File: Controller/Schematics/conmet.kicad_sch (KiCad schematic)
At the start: 14 parts, among them Q1 FQU20N06L, U1 RGBW_Led_Strip, U2 MP1584EN, U3 JS202011AQN, U4 VL53L1X

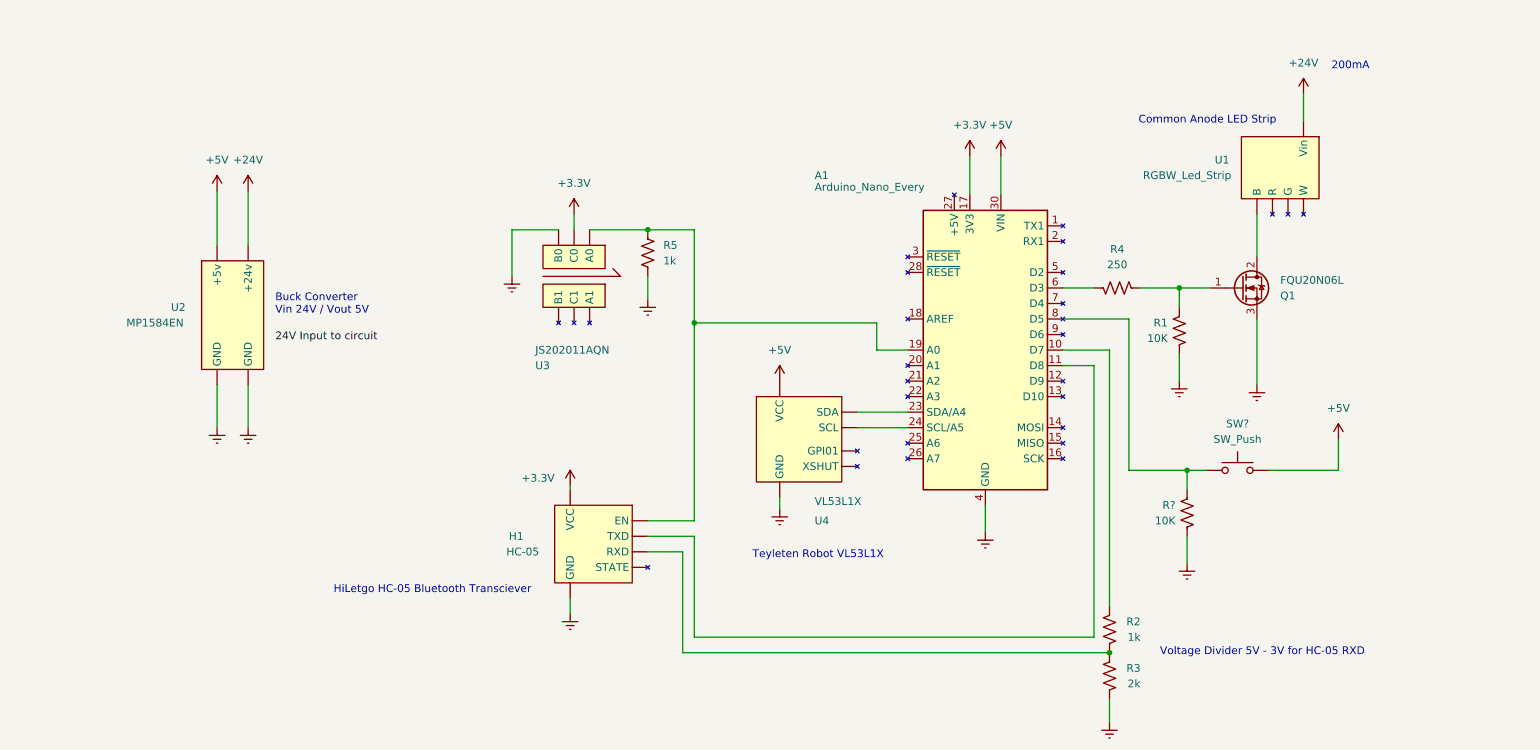
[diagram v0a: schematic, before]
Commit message: updates
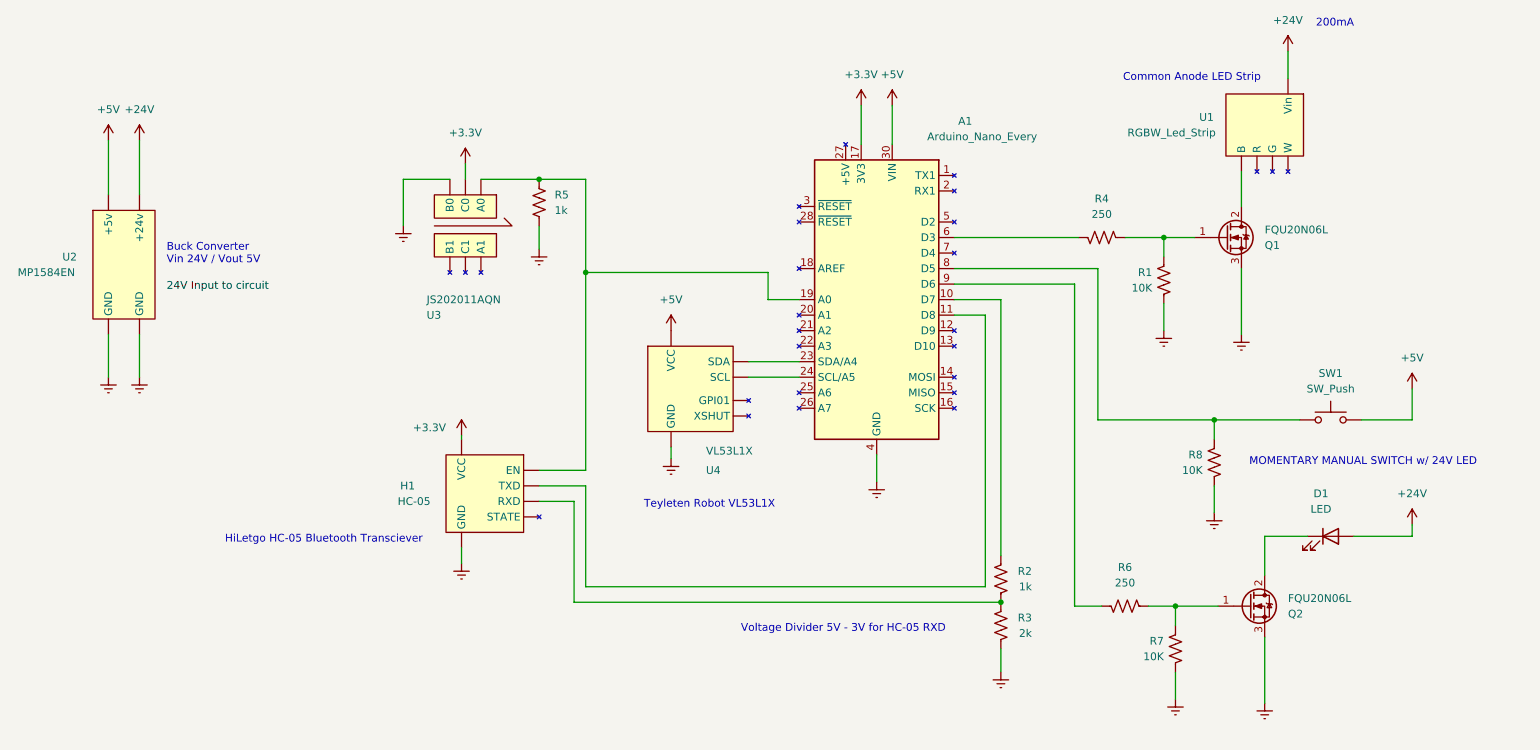
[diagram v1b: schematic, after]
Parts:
- added D1: LED, symbol Device:LED
- added Q2: FQU20N06L, symbol Device:Q_NMOS_DGS
- added R6: 250, symbol Device:R_US
- added R7: 10K, symbol Device:R_US
- gave numbers to parts that had none: 2
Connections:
- net +24V: now also D1.2 (A)
- net Earth: now also Q2.3 (S), R7.1
- net at A1.9 (D6): now also R6.2
- new net: Q2.1 (G), R6.1, R7.2
- new net: D1.1 (K), Q2.2 (D)
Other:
- note added: "MOMENTARY MANUAL SWITCH w/ 24V LED"
- moved on the sheet: H1, Q1, R1, R2, R3, R4, R5, R8, SW1, U1, U2, U3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
